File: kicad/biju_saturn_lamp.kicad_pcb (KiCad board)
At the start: 2 copper layers, 82.3 x 59.9 mm, 26 parts, among them J1 Barrel_Jack, J2 Conn_01x06, J3 Conn_01x02, J4 Conn_01x02, J5 Conn_01x02, SW1 SW_Push, U1 Pico, U2 74HC595, U3 PAM8302AAD

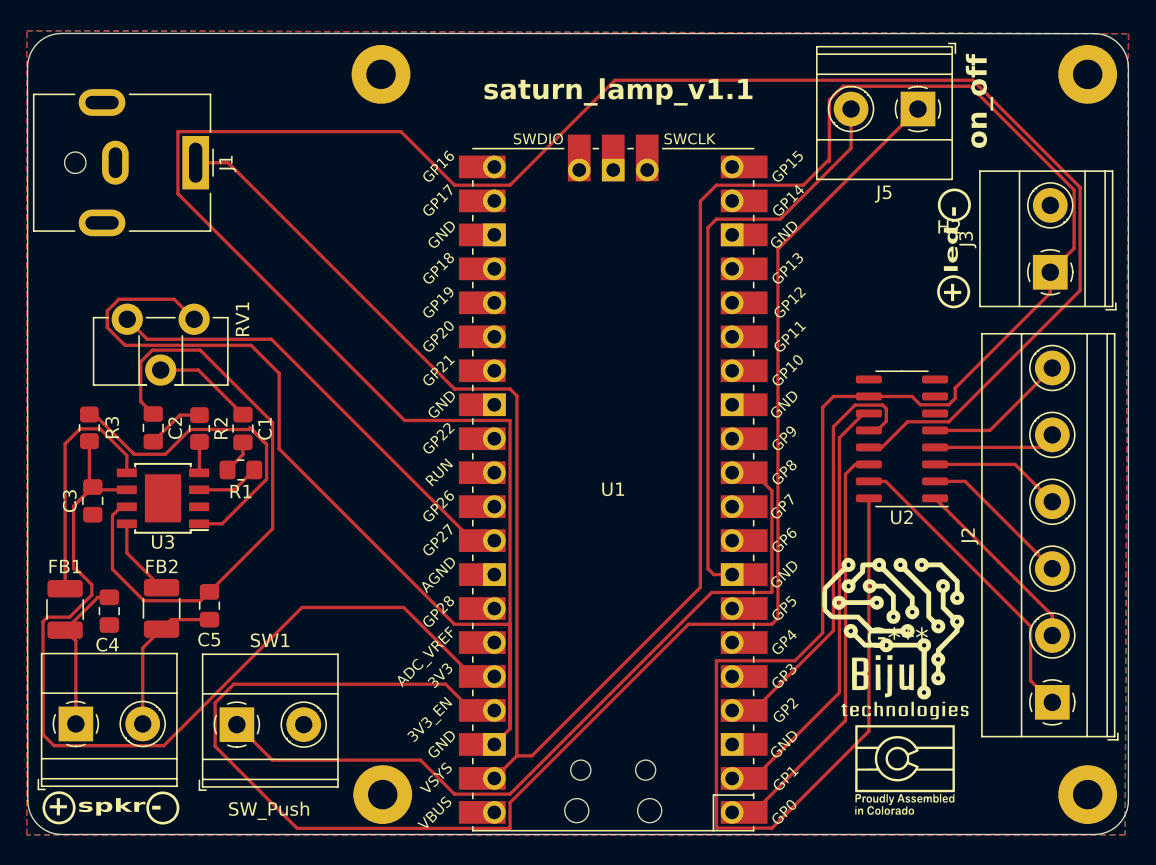
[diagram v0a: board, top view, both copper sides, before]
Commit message: update pcb
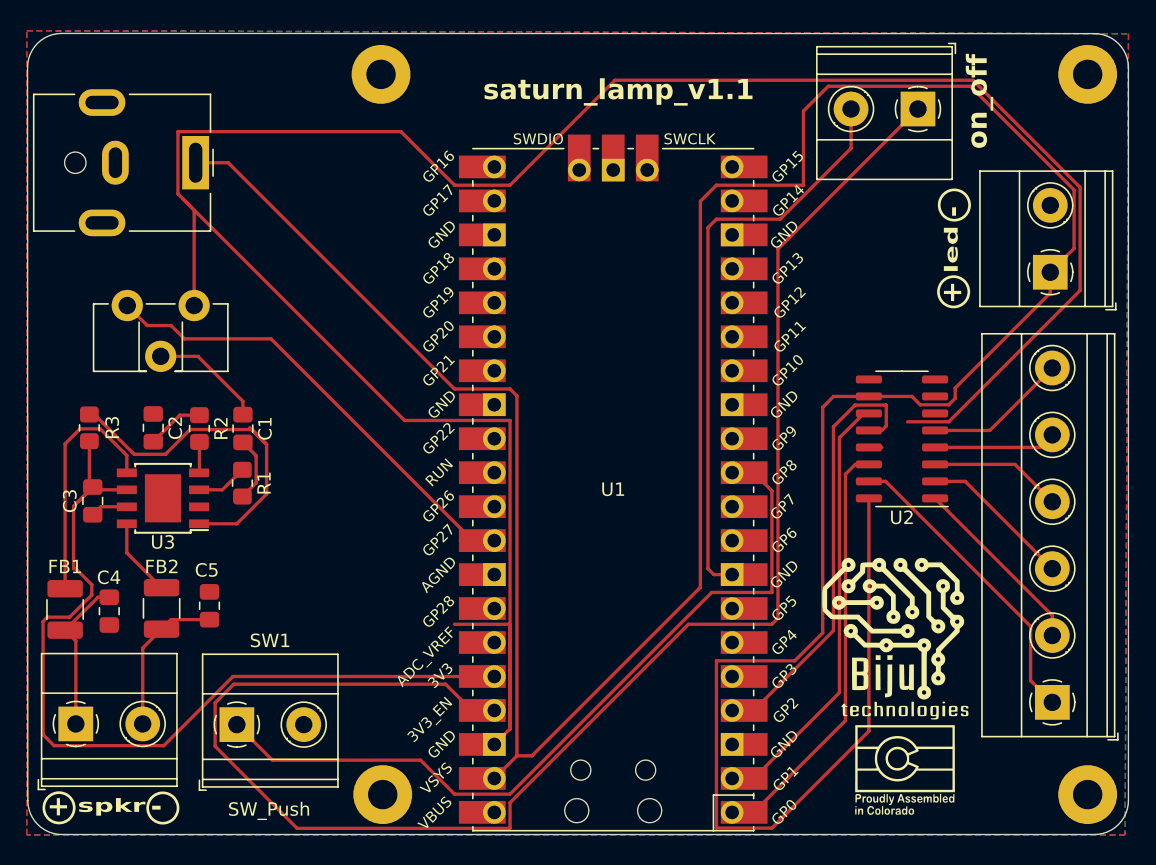
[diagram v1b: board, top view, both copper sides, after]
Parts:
- moved RV1 1.03 mm to (166.4, 99.1)
- moved R1 0.99 mm to (170.0, 112.3), turned to -90 degrees
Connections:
- U1 pad 18: unconnected-(U1-GND-Pad18) -> GND
- U1 pad 23: unconnected-(U1-GND-Pad23) -> GND
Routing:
- net GND: track 313.3 -> 229.3 mm
- net 3v3: track 70.5 -> 66.2 mm
- net Net-(C1-Pad2): track 2.54 -> 4.88 mm
- net Net-(C1-Pad1): track 7.53 -> 8.54 mm
- net Net-(U3-IN+): track 4.74 -> 3.86 mm
- net Net-(U3-~{SD}): track 26.5 -> 27.2 mm
